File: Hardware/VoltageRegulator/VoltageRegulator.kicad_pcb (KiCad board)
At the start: 2 copper layers, 22.1 x 14.2 mm, 10 parts, among them J1 Conn_01x04, U1 TPS7A2501DRVR

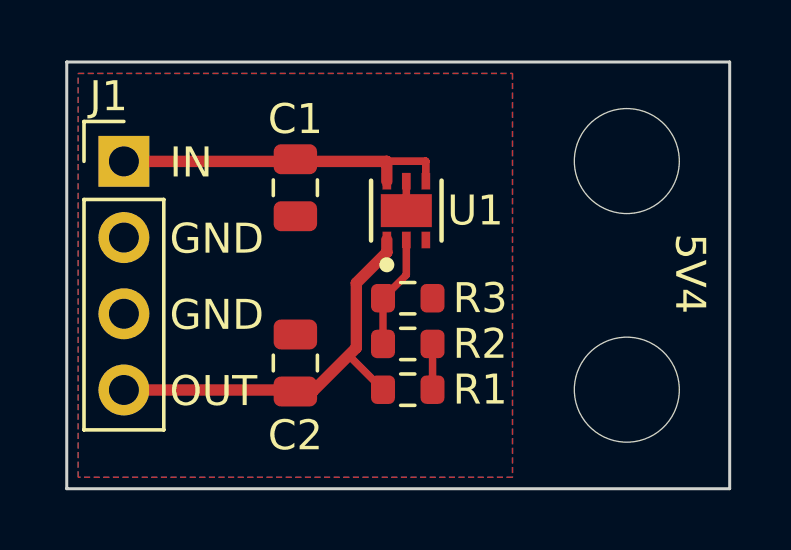
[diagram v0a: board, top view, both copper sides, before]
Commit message: Mmmmm...metric
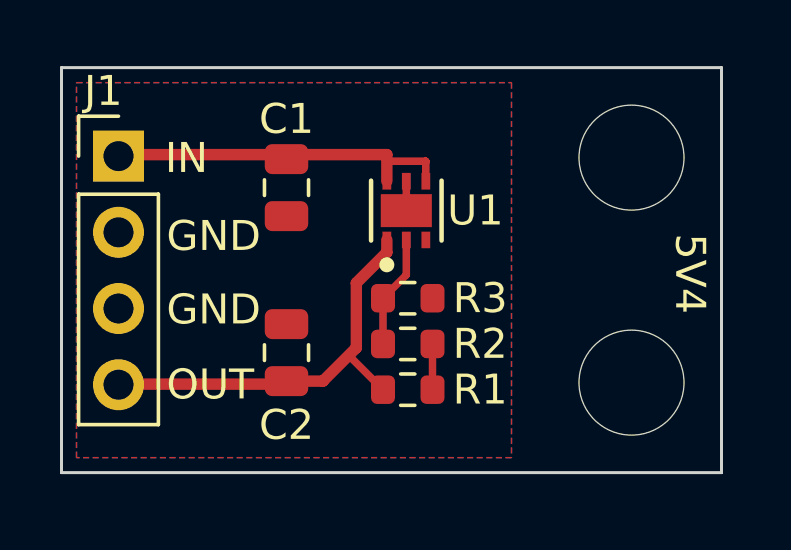
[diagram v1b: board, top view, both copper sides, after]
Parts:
- moved C2 0.45 mm to (137.5, 101.0)
- moved G*** 0.33 mm to (139.9, 98.3)
- moved C1 0.30 mm to (137.5, 95.5)
- moved H2 0.28 mm to (149.0, 102.0)
- moved J1 0.25 mm to (131.9, 94.5)
- moved H1 0.19 mm to (149.0, 94.5)
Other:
- board size 22.1 x 14.2 mm -> 22 x 13.5 mm
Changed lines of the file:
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@@
   (net 5 "Net-(U1-FB)")
   (footprint "Capacitor_SMD:C_0805_2012Metric" (layer "F.Cu")
-    (at 137.795 95.504 -90)
+    (at 137.5 95.5 -90)
     (descr "Capacitor SMD 0805 (2012 Metric), square (rectangular) end terminal, IPC_7351 nominal, (Body size source: IPC-SM-782 page 76, https://www.pcb-3d.com/wordpress/wp-content/uploads/ipc-sm-782a_amendment_1_and_2.pdf, https://docs.google.com/spreadsheets/d/1BsfQQcO9C6DZCsRaXUlFlo91Tg2WpOkGARC1WS5S8t0/edit?usp=sharing), generated with kicad-footprint-generator")
     (tags "capacitor")
@@
   )
   (footprint "Capacitor_SMD:C_0805_2012Metric" (layer "F.Cu")
-    (at 137.795 101.346 90)
+    (at 137.5 101 90)
     (descr "Capacitor SMD 0805 (2012 Metric), square (rectangular) end terminal, IPC_7351 nominal, (Body size source: IPC-SM-782 page 76, https://www.pcb-3d.com/wordpress/wp-content/uploads/ipc-sm-782a_amendment_1_and_2.pdf, https://docs.google.com/spreadsheets/d/1BsfQQcO9C6DZCsRaXUlFlo91Tg2WpOkGARC1WS5S8t0/edit?usp=sharing), generated with kicad-footprint-generator")
     (tags "capacitor")
@@
   )
   (footprint "MountingHole:MountingHole_3.5mm" (layer "F.Cu")
-    (at 148.844 94.615)
+    (at 149 94.5)
     (descr "Mounting Hole 3.5mm, no annular")
     (tags "mounting hole 3.5mm no annular")
@@
   )
   (footprint "Connector_PinHeader_2.54mm:PinHeader_1x04_P2.54mm_Vertical" (layer "F.Cu")
-    (at 132.08 94.625)
+    (at 131.9 94.45)
     (descr "Through hole straight pin header, 1x04, 2.54mm pitch, single row")
     (tags "Through hole pin header THT 1x04 2.54mm single row")
@@
   )
   (footprint "MountingHole:MountingHole_3.5mm" (layer "F.Cu")
-    (at 148.844 102.235)
+    (at 149 102)
     (descr "Mounting Hole 3.5mm, no annular")
     (tags "mounting hole 3.5mm no annular")
@@
   )
   (footprint "Clough42Logo:Clough42Logo" (layer "B.Cu")
-    (at 139.954 98.679 -90)
+    (at 139.95 98.35 -90)
     (attr board_only exclude_from_pos_files exclude_from_bom)
     (fp_text reference "G***" (at 0 0 90) (layer "B.SilkS") hide
@@
       (stroke (width 0) (type solid)) (fill solid) (layer "B.SilkS"))
   )
-  (gr_line (start 152.273 91.313) (end 152.273 105.537)
+  (gr_line (start 152 91.5) (end 152 105)
     (stroke (width 0.1) (type default)) (layer "Edge.Cuts"))
-  (gr_line (start 152.273 105.537) (end 130.175 105.537)
+  (gr_line (start 152 105) (end 130 105)
     (stroke (width 0.1) (type default)) (layer "Edge.Cuts"))
-  (gr_line (start 130.175 91.313) (end 152.273 91.313)
+  (gr_line (start 130 91.5) (end 152 91.5)
     (stroke (width 0.1) (type default)) (layer "Edge.Cuts"))
-  (gr_line (start 130.175 105.537) (end 130.175 91.313)
+  (gr_line (start 130 105) (end 130 91.5)
     (stroke (width 0.1) (type default)) (layer "Edge.Cuts"))
-  (gr_text "IN" (at 135.255 95.25) (layer "B.SilkS")
+  (gr_text "IN" (at 135.15 95.1) (layer "B.SilkS")
     (effects (font (size 1 1) (thickness 0.15)) (justify left bottom mirror))
   )
-  (gr_text "OUT" (at 136.652 102.87) (layer "B.SilkS")
+  (gr_text "OUT" (at 136.6 102.65) (layer "B.SilkS")
     (effects (font (size 1 1) (thickness 0.15)) (justify left bottom mirror))
   )
-  (gr_text "GND" (at 136.779 100.33) (layer "B.SilkS")
+  (gr_text "GND" (at 136.7 100.15) (layer "B.SilkS")
     (effects (font (size 1 1) (thickness 0.15)) (justify left bottom mirror))
   )
-  (gr_text "5V4 Regulator\n2023 v1.0" (at 144.399 98.552 90) (layer "B.SilkS")
+  (gr_text "5V4 Regulator\n2023 v1.0" (at 144.4 98.25 90) (layer "B.SilkS")
     (effects (font (size 1 1) (thickness 0.15)) (justify bottom mirror))
   )
-  (gr_text "GND" (at 136.779 97.79) (layer "B.SilkS")
+  (gr_text "GND" (at 136.7 97.65) (layer "B.SilkS")
     (effects (font (size 1 1) (thickness 0.15)) (justify left bottom mirror))
   )
-  (gr_text "GND" (at 133.604 97.79) (layer "F.SilkS")
+  (gr_text "GND" (at 133.5 97.7) (layer "F.SilkS")
     (effects (font (size 1 1) (thickness 0.15)) (justify left bottom))
   )
@@
     (effects (font (size 1 1) (thickness 0.15)) (justify left bottom))
   )
-  (gr_text "GND" (at 133.604 100.33) (layer "F.SilkS")
+  (gr_text "GND" (at 133.5 100.15) (layer "F.SilkS")
     (effects (font (size 1 1) (thickness 0.15)) (justify left bottom))
   )
-  (gr_text "IN" (at 133.604 95.25) (layer "F.SilkS")
+  (gr_text "IN" (at 133.45 95.1) (layer "F.SilkS")
     (effects (font (size 1 1) (thickness 0.15)) (justify left bottom))
   )
-  (gr_text "OUT" (at 133.604 102.87) (layer "F.SilkS")
+  (gr_text "OUT" (at 133.5 102.65) (layer "F.SilkS")
     (effects (font (size 1 1) (thickness 0.15)) (justify left bottom))
   )
   (dimension (type aligned) (layer "Dwgs.User")
-    (pts (xy 148.844 102.235) (xy 148.844 94.615))
+    (pts (xy 149 102) (xy 149 94.5))
     (height 10.668)
-    (gr_text "0.3000 in" (at 161.671 98.425 90) (layer "Dwgs.User")
+    (gr_text "7.5000 mm" (at 161.671 98.425 90) (layer "Dwgs.User")
       (effects (font (size 1.5 1.5) (thickness 0.3)))
     )
@@
   )
   (dimension (type aligned) (layer "Dwgs.User")
-    (pts (xy 130.175 91.313) (xy 130.175 105.537))
+    (pts (xy 130 91.5) (xy 130 105))
     (height 5.08)
-    (gr_text "0.5600 in" (at 123.295 98.425 90) (layer "Dwgs.User")
+    (gr_text "13.5000 mm" (at 123.12 98.25 90) (layer "Dwgs.User")
       (effects (font (size 1.5 1.5) (thickness 0.3)))
     )
@@
   )
   (dimension (type aligned) (layer "Dwgs.User")
-    (pts (xy 130.175 91.313) (xy 152.273 91.313))
+    (pts (xy 130 91.5) (xy 152 91.5))
     (height -2.413)
-    (gr_text "0.8700 in" (at 141.224 87.1) (layer "Dwgs.User")
+    (gr_text "22.0000 mm" (at 141 87.287) (layer "Dwgs.User")
       (effects (font (size 1.5 1.5) (thickness 0.3)))
     )
@@
     (style (thickness 0.2) (arrow_length 1.27) (text_position_mode 0) (extension_height 0.58642) (extension_offset 0.5) keep_text_aligned)
   )
-  (segment (start 132.08 94.625) (end 140.844 94.625) (width 0.381) (layer "F.Cu") (net 1))
   (segment (start 140.844 95.287968) (end 140.844 94.628935) (width 0.254) (layer "F.Cu") (net 1))
+  (segment (start 131.95 94.4) (end 140.844 94.4) (width 0.381) (layer "F.Cu") (net 1))
   (segment (start 142.144002 94.628935) (end 142.144002 95.287968) (width 0.254) (layer "F.Cu") (net 1))
   (segment (start 140.8535 94.619435) (end 142.134502 94.619435) (width 0.254) (layer "F.Cu") (net 1))
   (segment (start 140.844 94.628935) (end 140.8535 94.619435) (width 0.254) (layer "F.Cu") (net 1))
-  (segment (start 140.844 94.625) (end 140.844 95.287968) (width 0.381) (layer "F.Cu") (net 1))
+  (segment (start 140.844 94.4) (end 140.844 95.287968) (width 0.381) (layer "F.Cu") (net 1))
+  (segment (start 131.9 94.45) (end 131.95 94.4) (width 0.381) (layer "F.Cu") (net 1))
   (segment (start 142.134502 94.619435) (end 142.144002 94.628935) (width 0.254) (layer "F.Cu") (net 1))
   (segment (start 141.494001 95.287968) (end 141.494001 96.266) (width 0.25) (layer "F.Cu") (net 2))
+  (segment (start 139.827 98.679) (end 140.844 97.662) (width 0.381) (layer "F.Cu") (net 3))
   (segment (start 140.716 102.235) (end 139.5735 101.0925) (width 0.25) (layer "F.Cu") (net 3))
+  (segment (start 140.844 97.662) (end 140.844 97.244032) (width 0.381) (layer "F.Cu") (net 3))
+  (segment (start 138.716 101.95) (end 139.827 100.839) (width 0.381) (layer "F.Cu") (net 3))
+  (segment (start 137.5 101.95) (end 138.716 101.95) (width 0.381) (layer "F.Cu") (net 3))
+  (segment (start 137.4 102.05) (end 131.92 102.05) (width 0.381) (layer "F.Cu") (net 3))
   (segment (start 139.827 100.839) (end 139.827 98.679) (width 0.381) (layer "F.Cu") (net 3))
-  (segment (start 137.795 102.296) (end 138.37 102.296) (width 0.381) (layer "F.Cu") (net 3))
-  (segment (start 137.744 102.245) (end 132.08 102.245) (width 0.381) (layer "F.Cu") (net 3))
+  (segment (start 131.92 102.05) (end 131.9 102.07) (width 0.381) (layer "F.Cu") (net 3))
   (segment (start 140.717 102.235) (end 140.716 102.235) (width 0.25) (layer "F.Cu") (net 3))
-  (segment (start 137.795 102.296) (end 137.744 102.245) (width 0.381) (layer "F.Cu") (net 3))
-  (segment (start 139.827 98.679) (end 140.844 97.662) (width 0.381) (layer "F.Cu") (net 3))
-  (segment (start 138.37 102.296) (end 139.827 100.839) (width 0.381) (layer "F.Cu") (net 3))
-  (segment (start 140.844 97.662) (end 140.844 97.244032) (width 0.381) (layer "F.Cu") (net 3))
+  (segment (start 137.5 101.95) (end 137.4 102.05) (width 0.381) (layer "F.Cu") (net 3))
   (segment (start 142.367 102.235) (end 142.367 100.711) (width 0.25) (layer "F.Cu") (net 4))
   (segment (start 140.717 100.711) (end 140.717 99.187) (width 0.25) (layer "F.Cu") (net 5))
@@
     (polygon
       (pts
-        (xy 145.034 91.694)
-        (xy 145.034 105.156)
-        (xy 130.556 105.156)
-        (xy 130.556 91.694)
+        (xy 145 92)
+        (xy 145 104.5)
+        (xy 130.5 104.5)
+        (xy 130.5 92)
       )
     )
@@
     (polygon
       (pts
-        (xy 130.556 91.694)
-        (xy 145.034 91.694)
-        (xy 145.034 105.156)
-        (xy 130.556 105.156)
-      )
-    )
+        (xy 130.5 92)
+        (xy 145 92)
+        (xy 145 104.5)
+        (xy 130.5 104.5)
+      )
+    )
